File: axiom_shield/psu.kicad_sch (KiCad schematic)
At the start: 6 parts, among them J1 USB_C_Receptacle_USB2.0_14P, U1 USBLC6-2P6

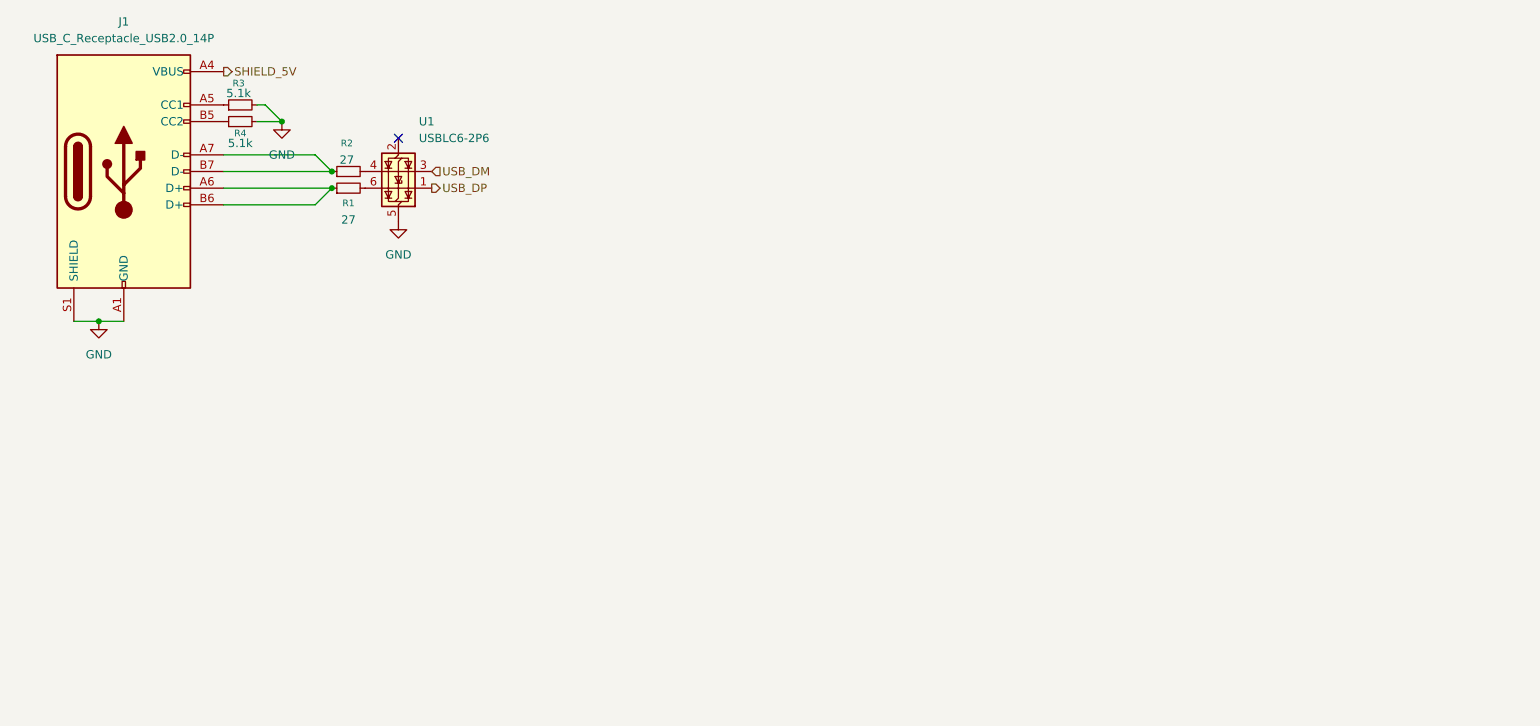
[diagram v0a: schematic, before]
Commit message: upload
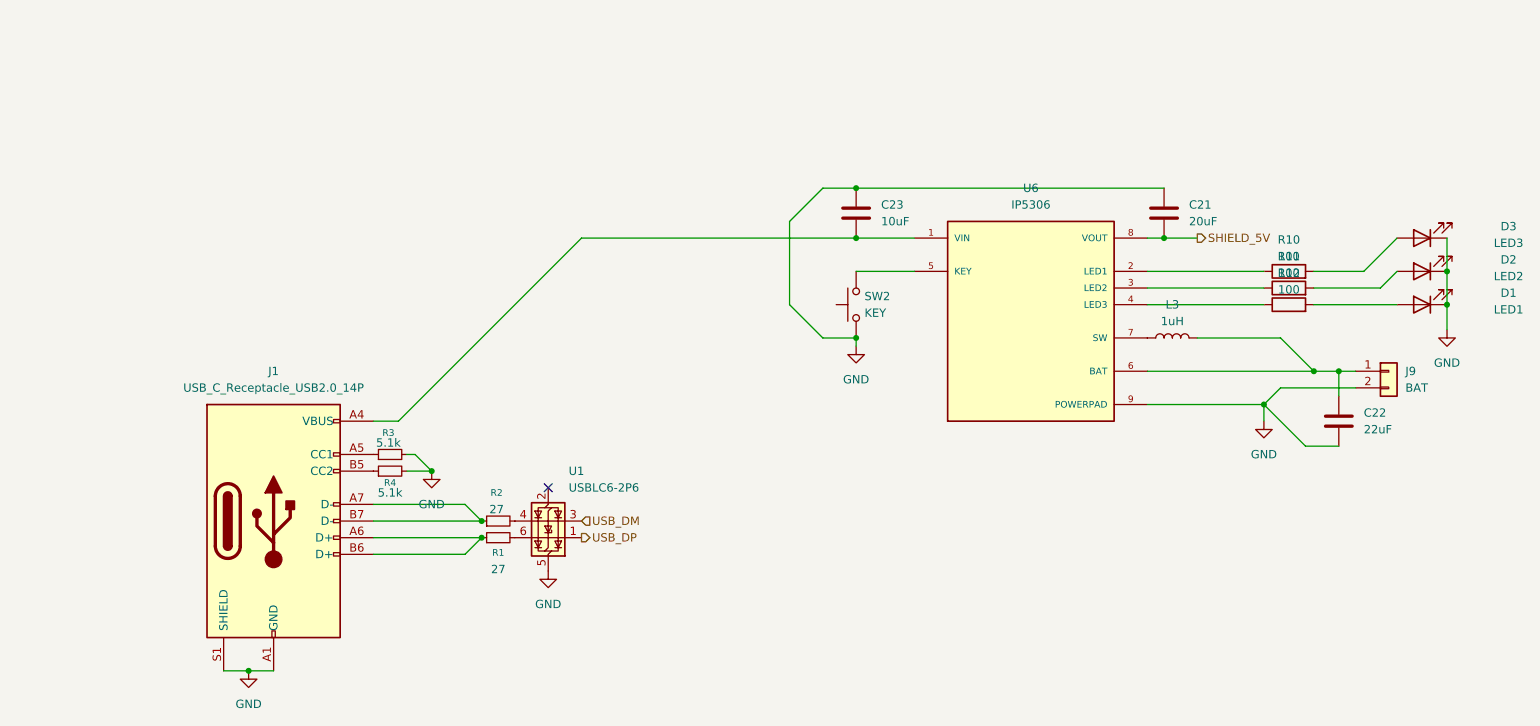
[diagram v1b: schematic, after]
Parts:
- added C21: 20uF, symbol Device:C
- added C22: 22uF, symbol Device:C
- added C23: 10uF, symbol Device:C
- added D1: LED1, symbol Device:LED
- added D2: LED2, symbol Device:LED
- added D3: LED3, symbol Device:LED
- added J9: BAT, symbol Connector_Generic:Conn_01x02
- added L3: 1uH, symbol Device:L
- added R10, R11, R12: 100, symbol Device:R
- added SW2: KEY, symbol Switch:SW_Push
- added U6: IP5306, IP5306:SOP127P600X165-9N, symbol IP5306:IP5306
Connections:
- net GND: now also C21.1, C22.2, C23.1, D1.1 (K), D2.1 (K), D3.1 (K), J9.2 (Pin_2), SW2.1, U6.9 (POWERPAD)
- net SHIELD_5V: now also C21.2, U6.8 (VOUT); no longer J1.A4 (VBUS), J1.A9 (VBUS), J1.B4 (VBUS), J1.B9 (VBUS)
- new net: D3.2 (A), R10.2
- new net: C22.1, J9.1 (Pin_1), L3.2, U6.6 (BAT)
- new net: D1.2 (A), R12.2
- new net: R10.1, U6.2 (LED1)
- new net: D2.2 (A), R11.2
- new net: SW2.2, U6.5 (KEY)
- new net: C23.2, J1.A4 (VBUS), J1.A9 (VBUS), J1.B4 (VBUS), J1.B9 (VBUS), U6.1 (VIN)
- new net: L3.1, U6.7 (SW)
- new net: R12.1, U6.4 (LED3)
- new net: R11.1, U6.3 (LED2)
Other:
- moved on the sheet: J1, R1, R2, R3, R4, U1
